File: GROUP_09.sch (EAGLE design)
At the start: 29 parts, among them J1 POWER_JACKPTH_LOCK, U1 +12v, U3 TCA9546ATSSOP16, U4 TMUX1208QNF

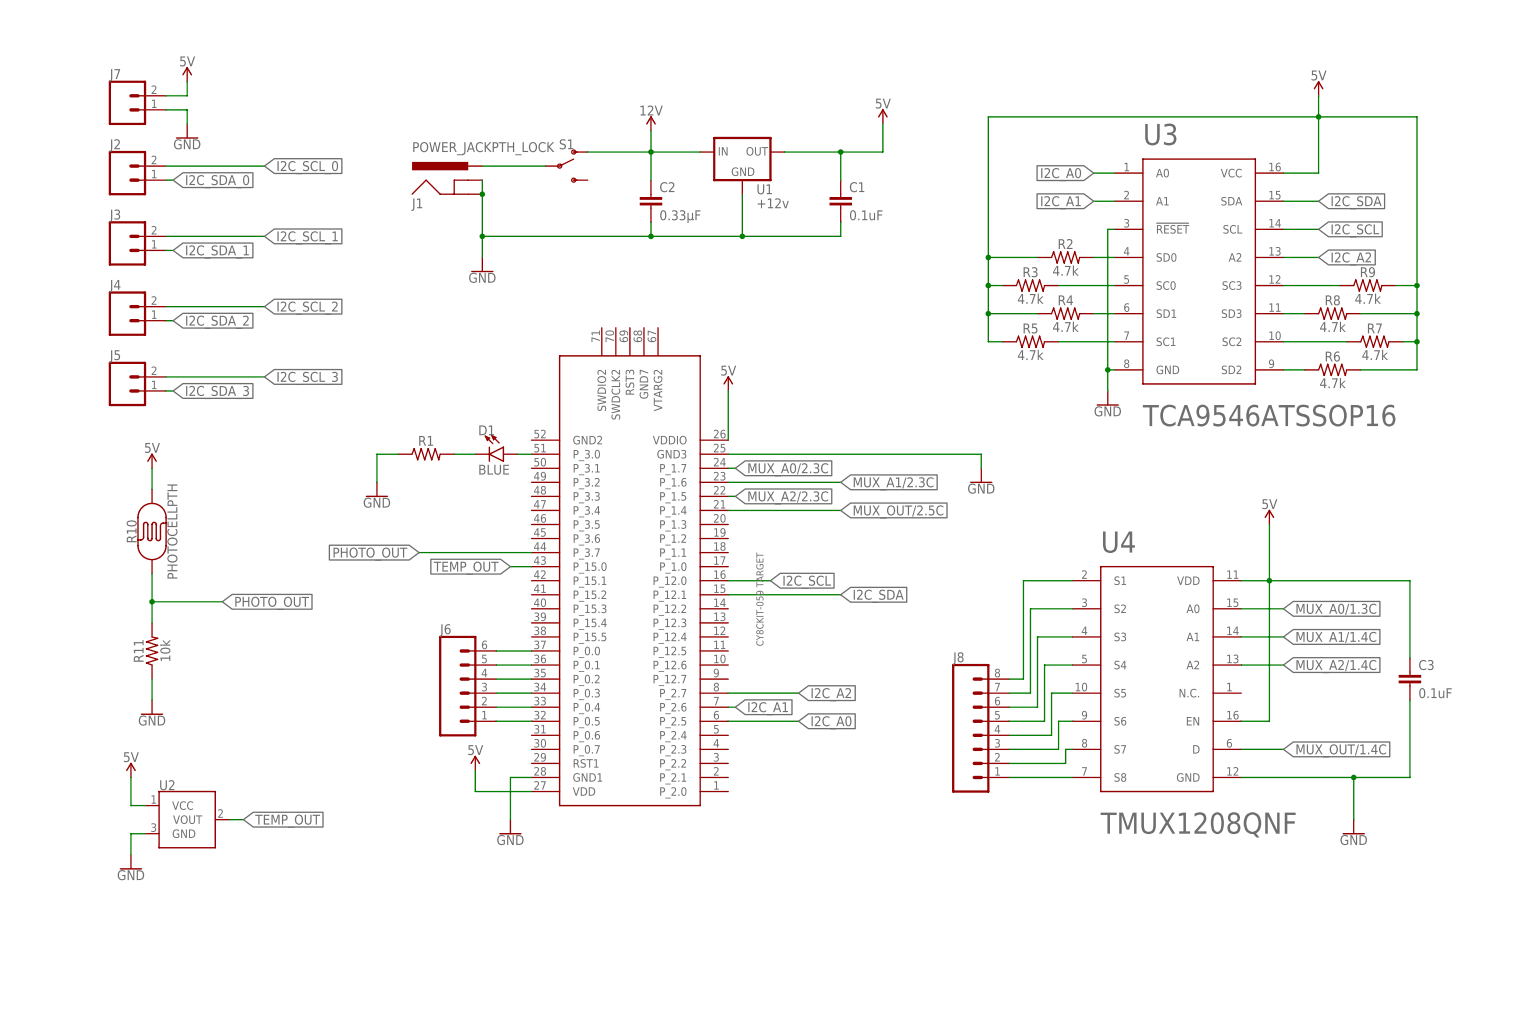
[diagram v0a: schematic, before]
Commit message: Final version
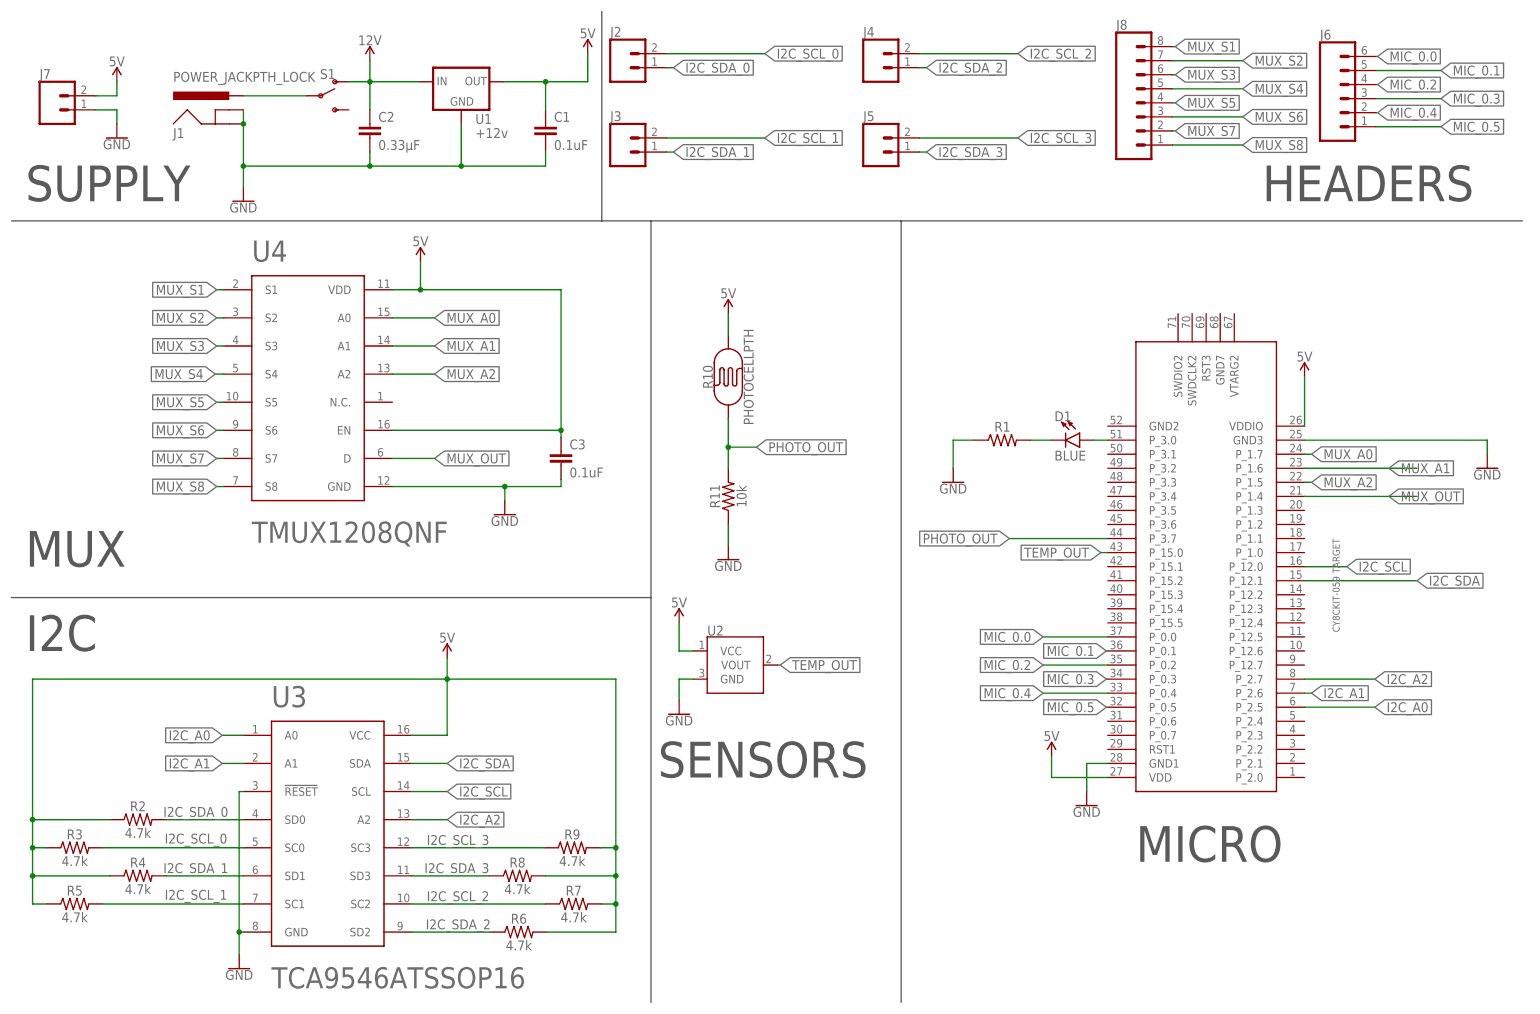
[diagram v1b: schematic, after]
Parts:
- J2, J3, J4, J5, J6, J7, J8, S1, U2: value (none) -> (none)
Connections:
- net N$12 renamed MIC_0.5
- net N$13 renamed MIC_0.4
- net N$14 renamed MIC_0.3
- net N$15 renamed MIC_0.2
- net N$16 renamed MIC_0.1
- net N$17 renamed MIC_0.0
- net N$18 renamed MUX_S8
- net N$19 renamed MUX_S7
- net N$20 renamed MUX_S6
- net N$21 renamed MUX_S5
- net N$22 renamed MUX_S4
- net N$23 renamed MUX_S3
- net N$24 renamed MUX_S2
- net N$25 renamed MUX_S1
- removed net MUX_A0/1.3C: U4.A0
- removed net MUX_A0/2.3C: CY8CKIT059-TARGET.P_1.7
- removed net MUX_A1/1.4C: U4.A1
- removed net MUX_A1/2.3C: CY8CKIT059-TARGET.P_1.6
- removed net MUX_A2/1.4C: U4.A2
- removed net MUX_A2/2.3C: CY8CKIT059-TARGET.P_1.5
- removed net MUX_OUT/1.4C: U4.D
- removed net MUX_OUT/2.5C: CY8CKIT059-TARGET.P_1.4
- removed net N$1: R2.2, U3.SD0
- removed net N$10: R6.1, U3.SD2
- removed net N$3: R3.2, U3.SC0
- removed net N$4: R4.2, U3.SD1
- removed net N$5: R5.2, U3.SC1
- removed net N$7: R9.1, U3.SC3
- removed net N$8: R8.1, U3.SD3
- removed net N$9: R7.1, U3.SC2
- new net MUX_A0: CY8CKIT059-TARGET.P_1.7, U4.A0
- new net MUX_A1: CY8CKIT059-TARGET.P_1.6, U4.A1
- new net MUX_A2: CY8CKIT059-TARGET.P_1.5, U4.A2
- new net MUX_OUT: CY8CKIT059-TARGET.P_1.4, U4.D
- net I2C_SCL_0: now also R3.2, U3.SC0
- net I2C_SCL_1: now also R5.2, U3.SC1
- net I2C_SCL_2: now also R7.1, U3.SC2
- net I2C_SCL_3: now also R9.1, U3.SC3
- net I2C_SDA_0: now also R2.2, U3.SD0
- net I2C_SDA_1: now also R4.2, U3.SD1
- net I2C_SDA_2: now also R6.1, U3.SD2
- net I2C_SDA_3: now also R8.1, U3.SD3
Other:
- note added: "HEADERS"
- note added: "I2C"
- note added: "MICRO"
- note added: "MUX"
- note added: "SENSORS"
- note added: "SUPPLY"
- moved on the sheet: C1, C2, C3, D1, J1, J2, J3, J4, J5, J6, J7, J8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
